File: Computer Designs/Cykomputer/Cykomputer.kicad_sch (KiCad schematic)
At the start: 64 parts, among them J1 Bus_ISA_8bit, J10 DE15_Socket_HighDensity_Mount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, J12 IEC_60320_C14_Receptacle, J13 Conn_01x02, J14 PINHD_1x2_Male, J15 Bus_ISA_8bit, J16 Conn_02x12_Row_Letter_First, J17 Conn_01x12, J2 Bus_ISA_8bit, J3 Bus_ISA_8bit, J4 DE9_Pins_MountingHoles, J5 DE9_Pins_MountingHoles, J6 Mini-DIN-6, J7 DE15_Socket_HighDensity_Mount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, J8 DE15_Socket_HighDensity_Mount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, J9 DE15_Socket_HighDensity_Mount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, P1 USB_C_Plug_USB2.0, SW1 SW_SPST, SW2 SW_Rotary_1x7_MP, U1 W65C02SxP, U10 74HC14, U12 W65C02SxP, U13 27C256, U14 KM62256CLP, U15 KM62256CLP, U16 27C256, U17 74HCT595, U18 74HCT164, U19 KM62256CLP, U2 W65C22SxP, U22 W65C22SxP, U23 74HCT595, U24 74HCT595, U25 KM62256CLP, U26 W65C22SxP, U3 W65C22SxP, U4 W65C22SxP, U5 W65C51NxP, U6 W65C51NxP, U7 MAX232, U8 MAX232, U9 W65C22SxP, Y1 ACO-xxxMHz-A, Y2 ACO-xxxMHz-A, Y3 ACO-xxxMHz-A, Y4 ACO-xxxMHz-A, Y5 ACO-xxxMHz-A, Y6 ACO-xxxMHz-A, Y7 ACO-xxxMHz-A

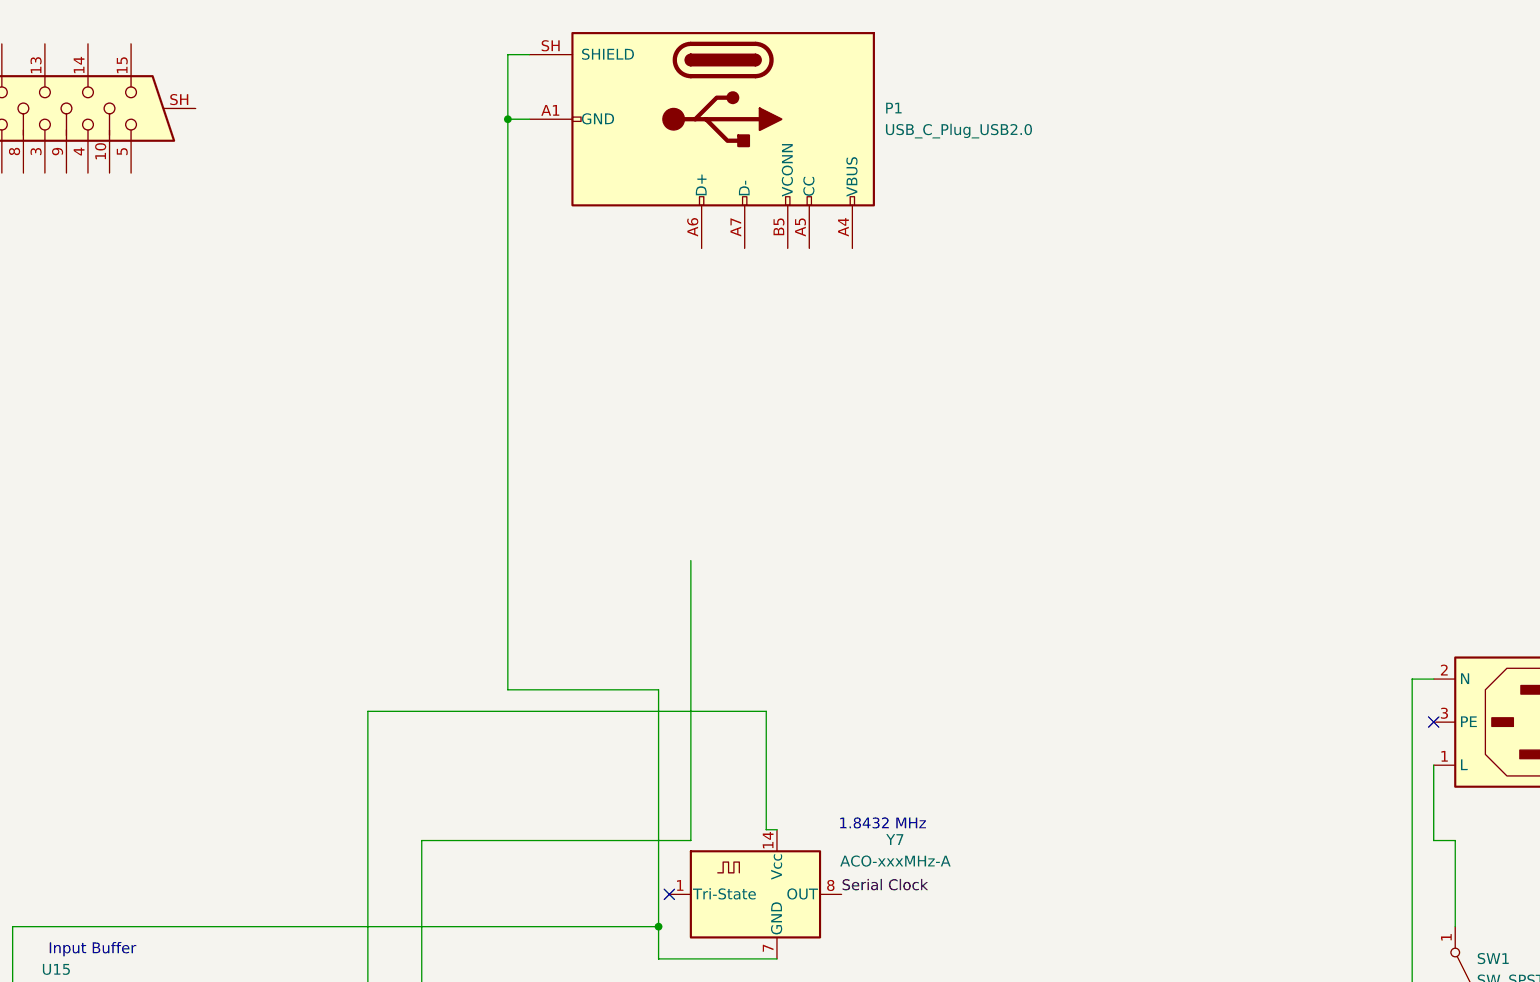
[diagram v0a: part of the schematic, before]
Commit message: Updated Computer schematic
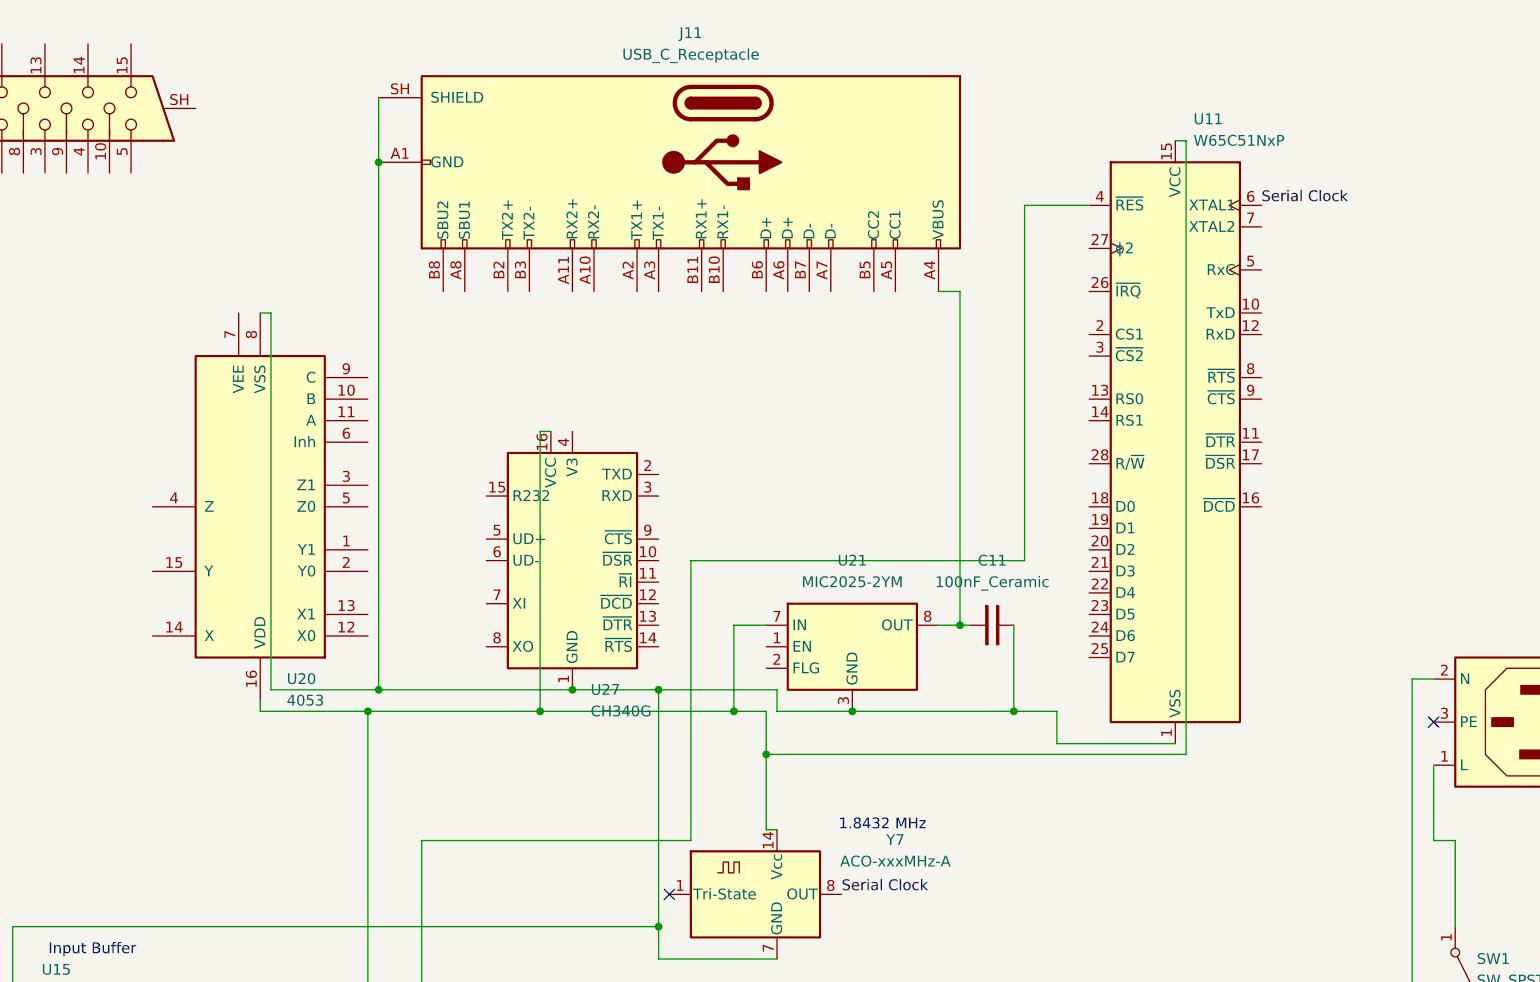
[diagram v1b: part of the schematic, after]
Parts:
- removed P1: USB_C_Plug_USB2.0, symbol Connector:USB_C_Plug_USB2.0
- added C11: 100nF_Ceramic, Capacitor_THT:C_Disc_D5.0mm_W2.5mm_P2.50mm, symbol PCM_SL_Capacitors:100nF_Ceramic
- added J11: USB_C_Receptacle, symbol Connector:USB_C_Receptacle
- added U11: W65C51NxP, Package_DIP:DIP-28_W15.24mm, symbol PCM_65xx-library:W65C51NxP
- added U20: 4053, symbol 4xxx:4053
- added U21: MIC2025-2YM, Package_SO:SOIC-8_3.9x4.9mm_P1.27mm, symbol Power_Management:MIC2025-2YM
- added U27: CH340G, Package_SO:SOIC-16_3.9x9.9mm_P1.27mm, symbol Interface_USB:CH340G
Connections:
- net GND: now also C11.2, J11.A1 (GND), J11.A12 (GND), J11.B1 (GND), J11.B12 (GND), J11.SH (SHIELD), U11.1 (VSS), U20.8 (VSS), U21.3 (GND), U27.1 (GND)
- net Serial Clock: now also U11.6 (XTAL1)
- net VCC: now also U11.15 (VCC), U20.16 (VDD), U21.7 (IN), U27.16 (VCC)
- net at SW2.8, U1.39 (ϕ2), U5.27 (ϕ2)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: now also U11.4 (~{RES})
- new net: C11.1, J11.A4 (VBUS), J11.A9 (VBUS), J11.B4 (VBUS), J11.B9 (VBUS), U21.6 (OUT), U21.8 (OUT)
